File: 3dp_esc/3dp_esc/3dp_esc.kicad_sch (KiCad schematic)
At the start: 14 parts, among them J1 Conn_01x03_Pin, J2 Conn_01x02_Pin, U1 NE555P

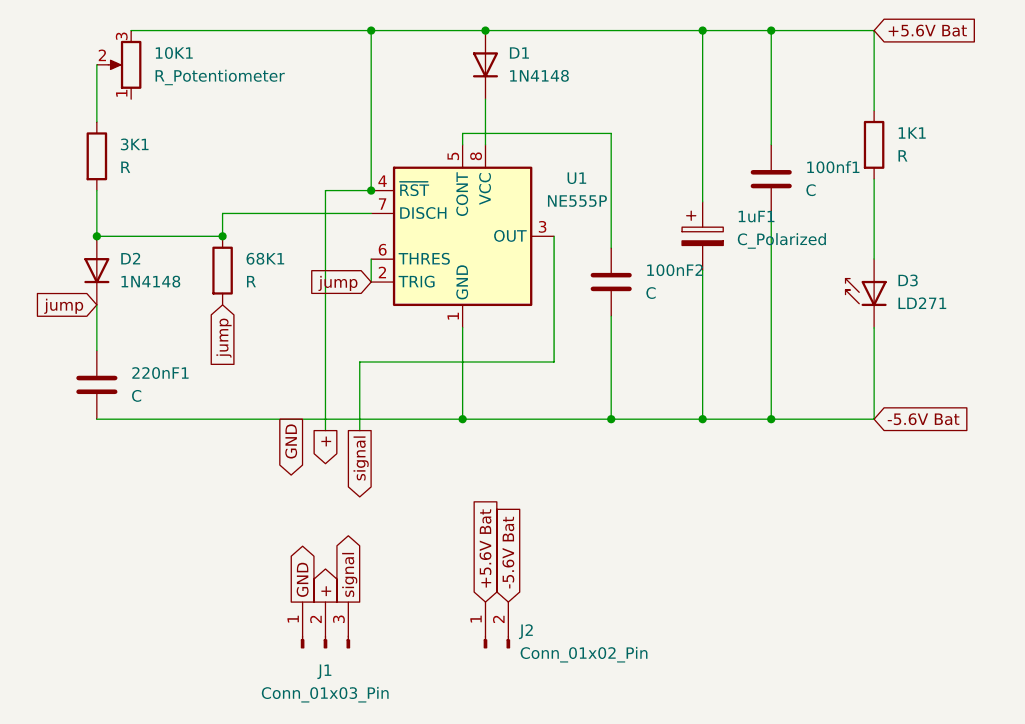
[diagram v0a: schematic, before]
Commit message: this is good
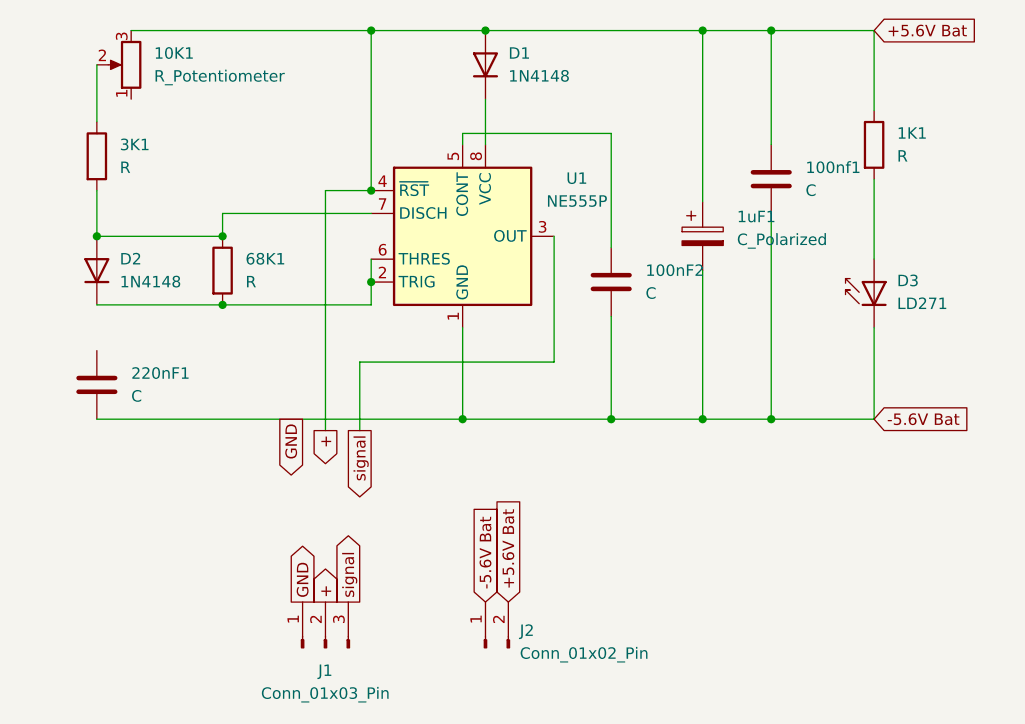
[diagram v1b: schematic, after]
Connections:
- net +: now also J2.2 (Pin_2); no longer J2.1 (Pin_1)
- net -5.6V Bat: now also J2.1 (Pin_1); no longer J2.2 (Pin_2)
- net jump: no longer names the net of 68K1.2, D2.1 (K), U1.2 (TRIG), U1.6 (THRES)
- net jump: no longer 220nF1.1
